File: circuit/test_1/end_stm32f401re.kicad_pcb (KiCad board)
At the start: 2 copper layers, 73.9 x 76 mm, 27 parts, among them J1 Micro_SD_Card_Det, J2 USB_B_Micro, U1 MAX98357_DAC, U2 NUCLEO-64

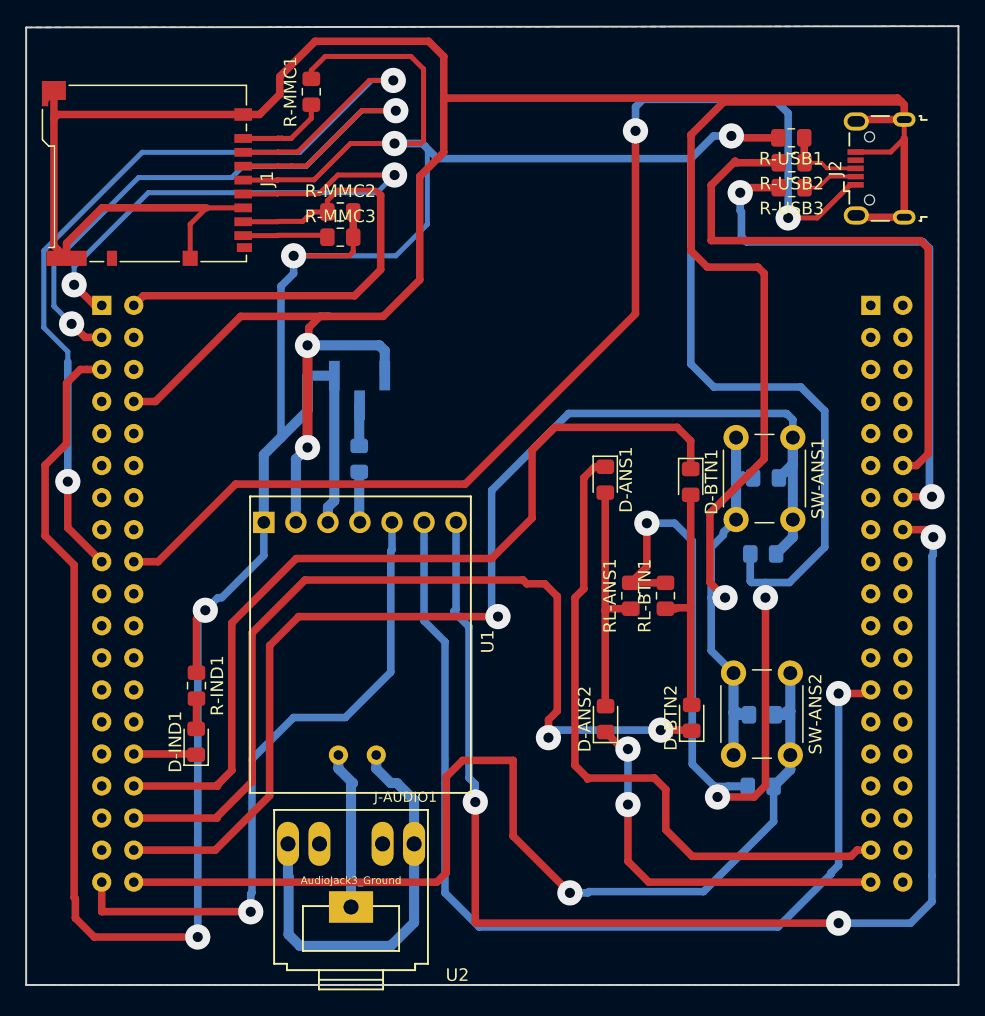
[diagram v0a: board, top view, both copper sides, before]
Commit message: PCB board and test
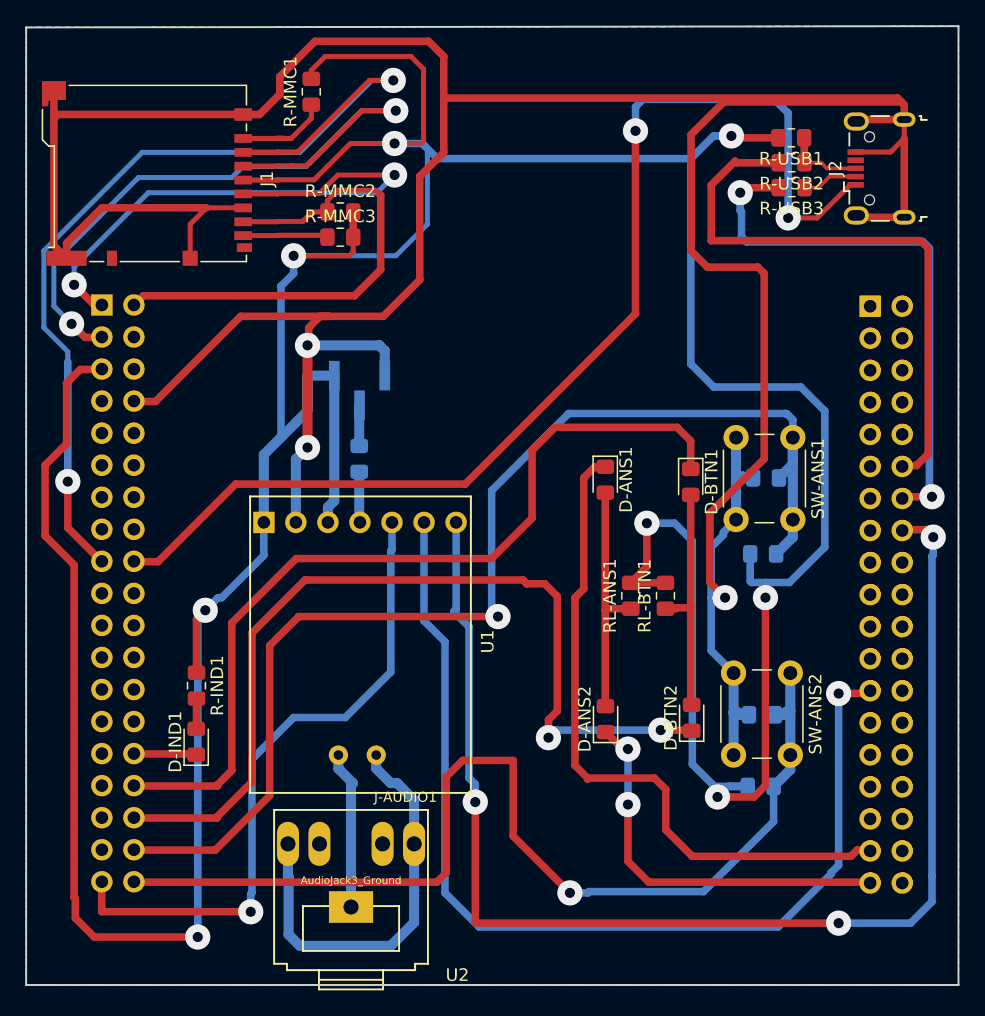
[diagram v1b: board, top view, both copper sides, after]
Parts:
- added J-Shield1: Conn_02x19_Odd_Even, Connector_PinSocket_2.54mm:PinSocket_2x19_P2.54mm_Vertical, B.Cu at (110.4, 86.3)
- added J-Shield2: Conn_02x19_Odd_Even, Connector_PinSocket_2.54mm:PinSocket_2x19_P2.54mm_Vertical, B.Cu at (171.3, 86.4)
